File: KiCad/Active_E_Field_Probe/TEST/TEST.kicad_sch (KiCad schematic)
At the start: 91 parts

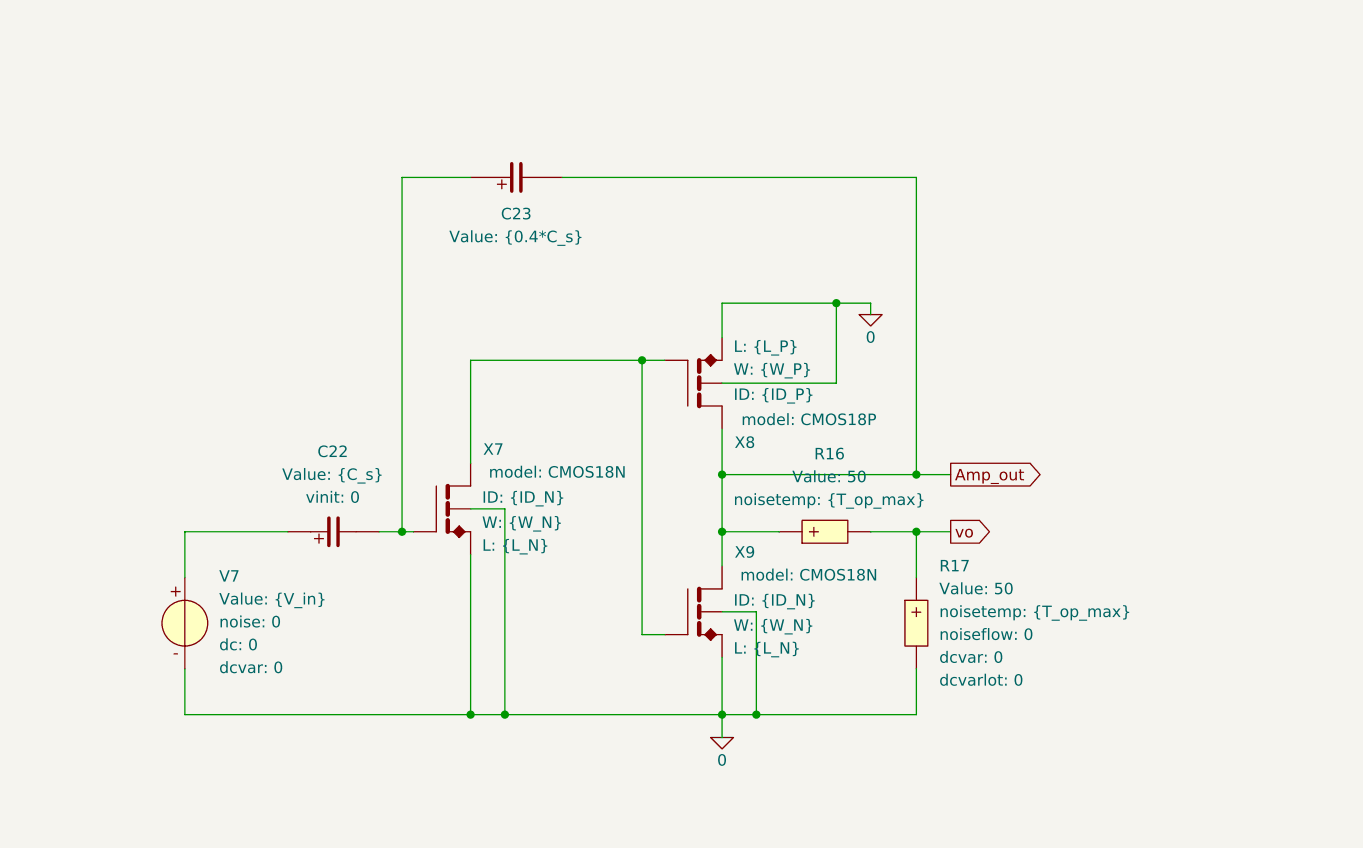
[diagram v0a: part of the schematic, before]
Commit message: something
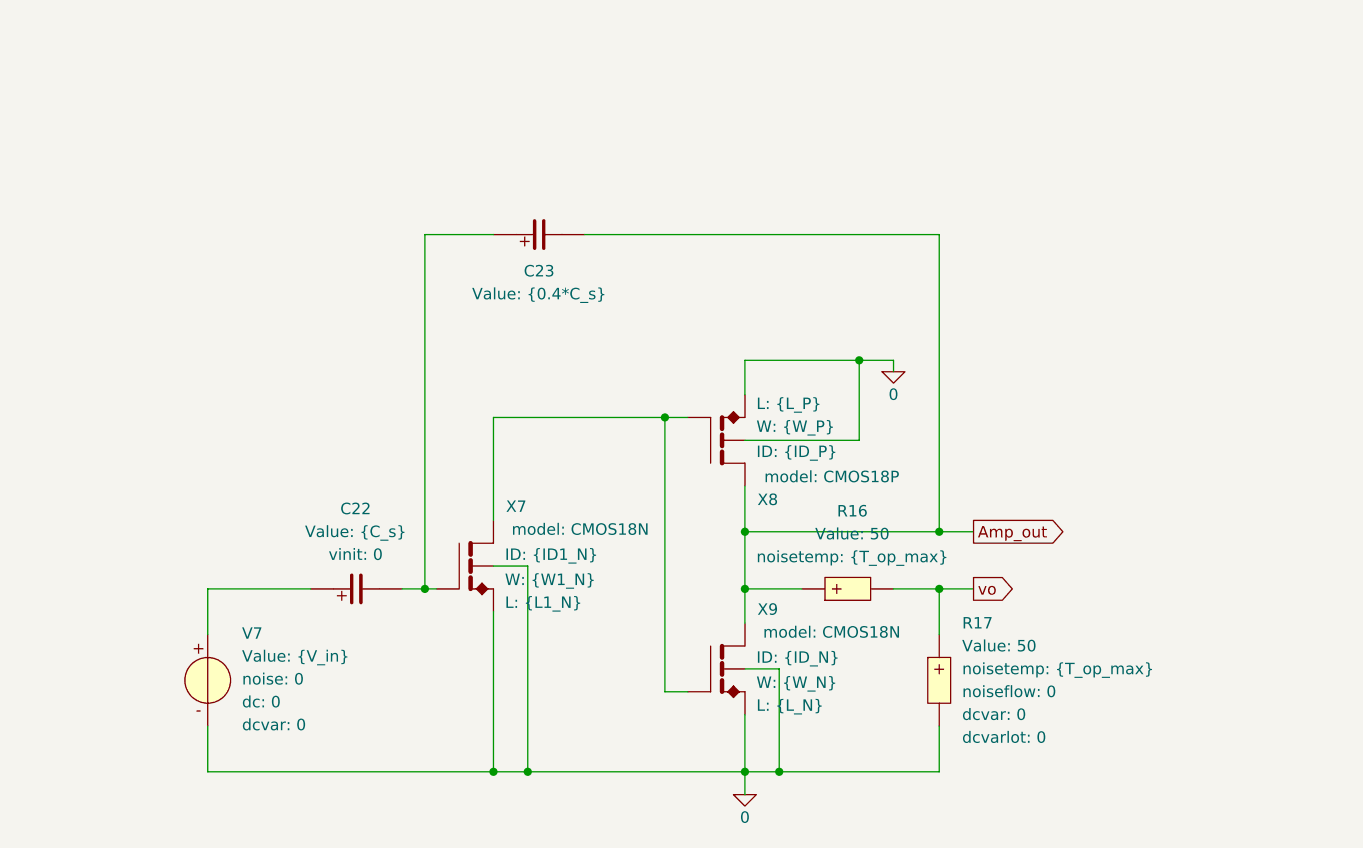
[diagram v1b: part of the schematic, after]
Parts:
- X7: ID {ID_N} -> {ID1_N}; L {L_N} -> {L1_N}; W {W_N} -> {W1_N}
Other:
- moved on the sheet: C22, C23, R16, R17

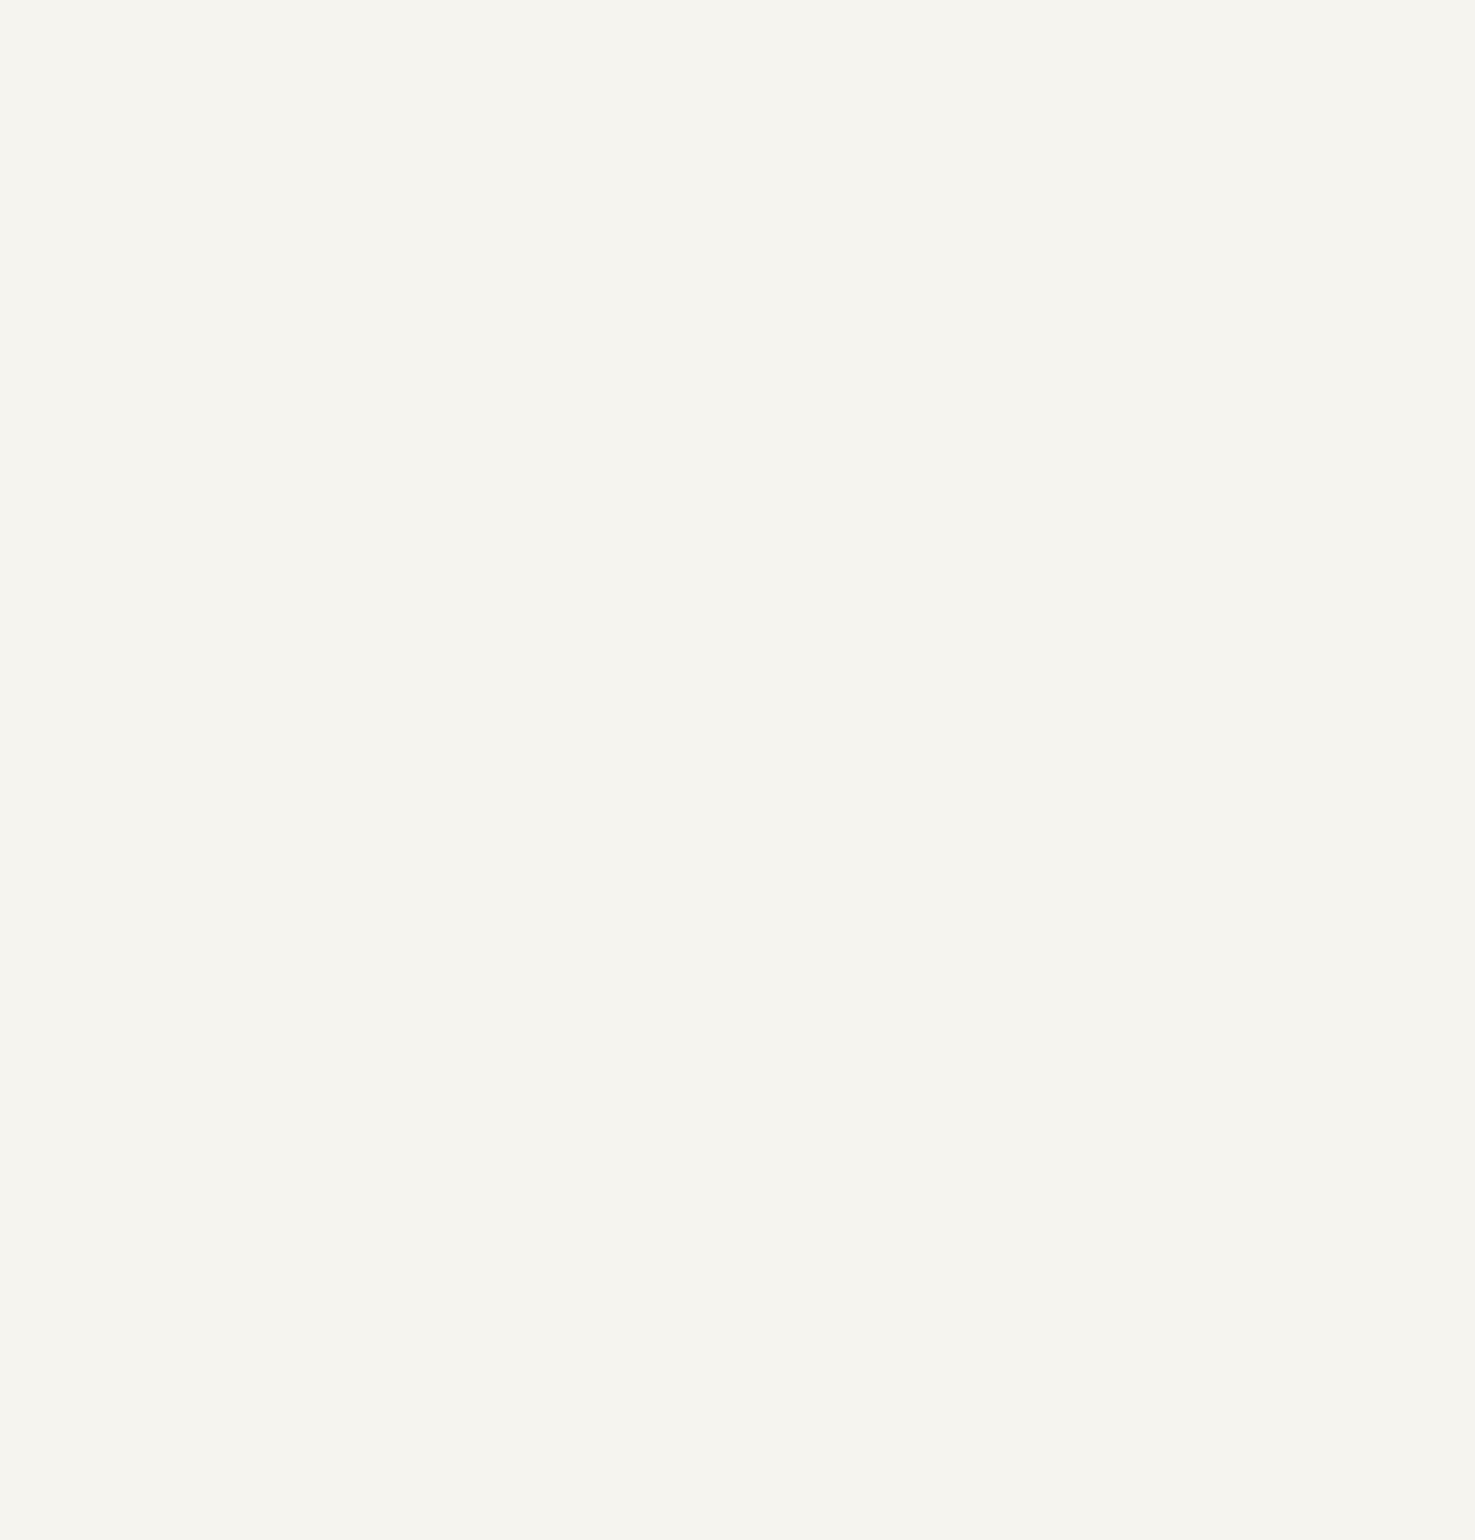
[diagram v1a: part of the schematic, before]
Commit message: Loopgain Fucked
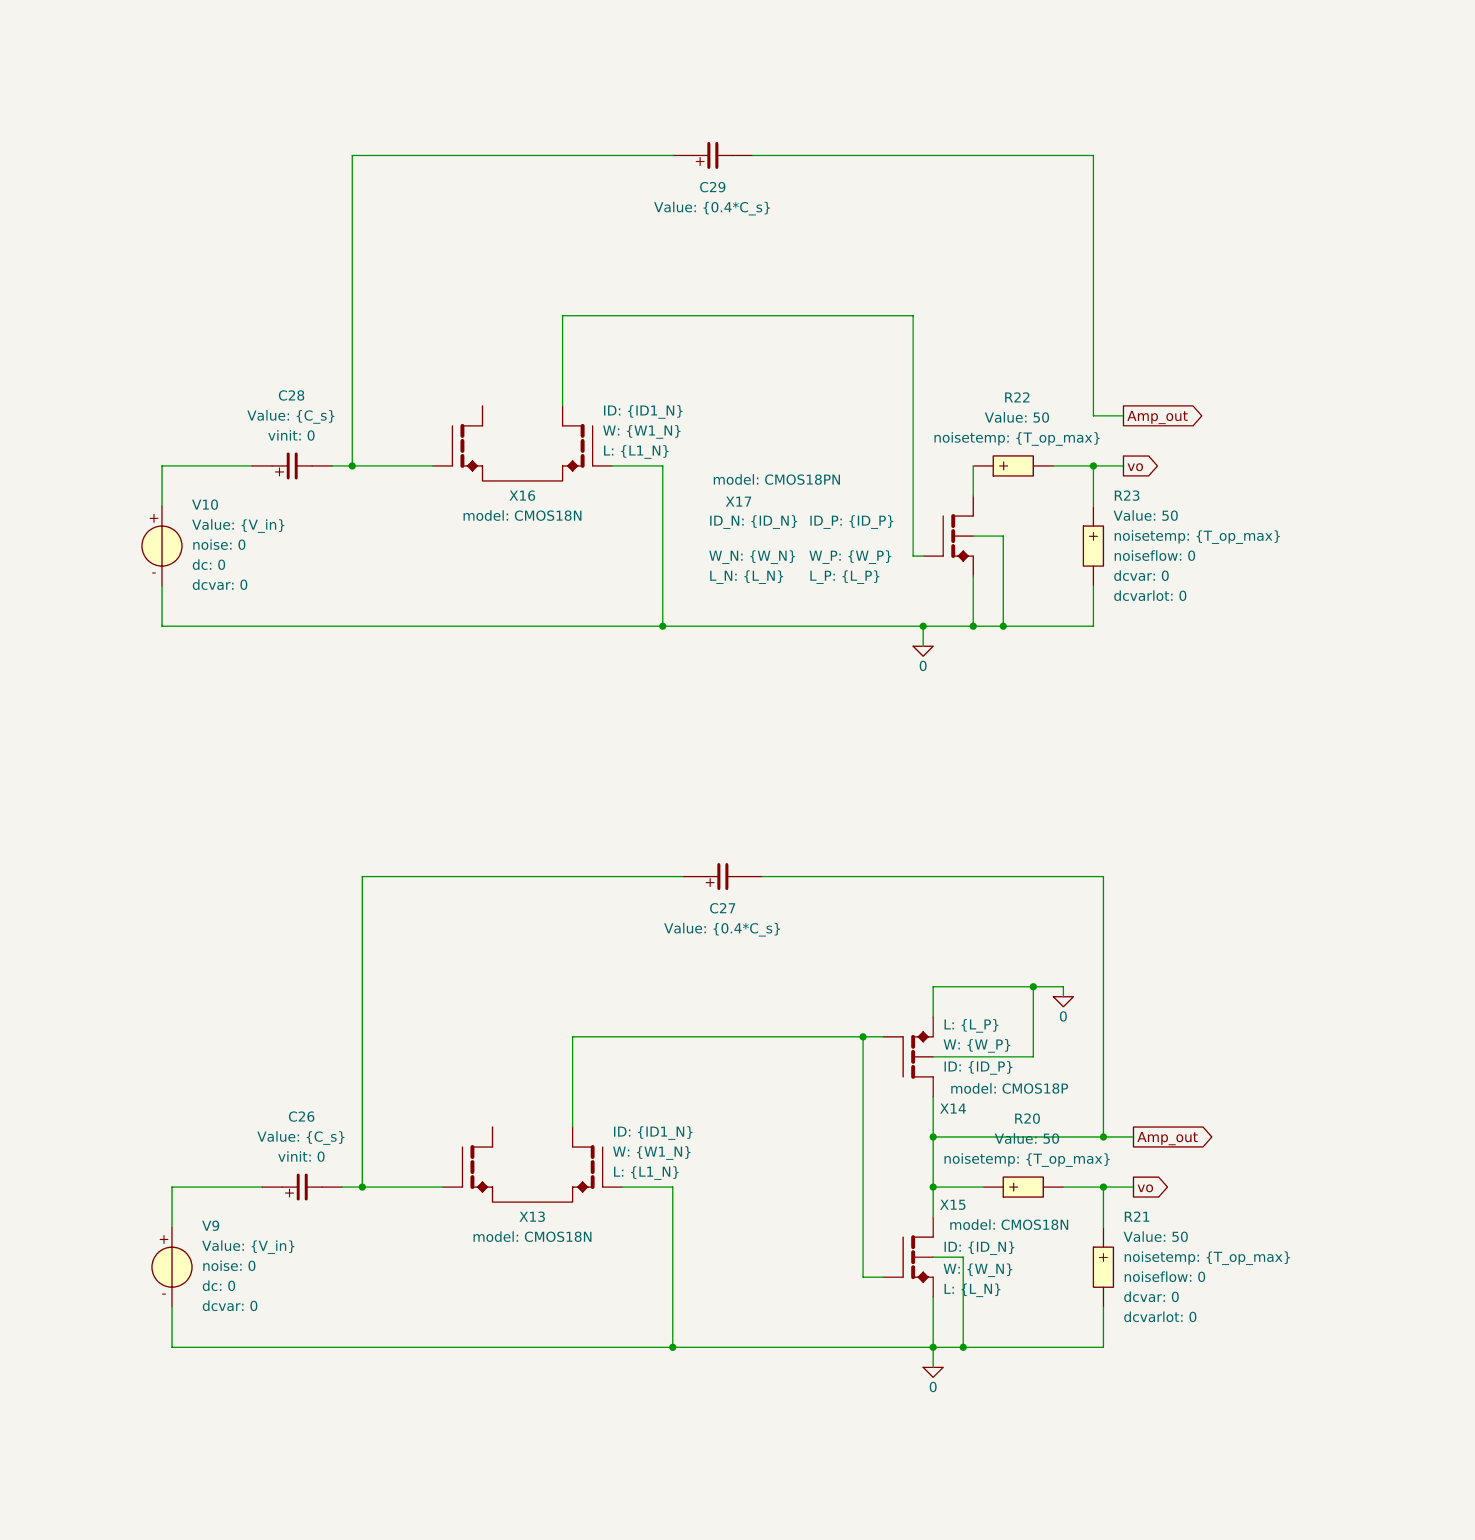
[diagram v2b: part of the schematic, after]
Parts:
- added C26, C28: {C_s}, symbol SLiCAP:C
- added C27, C29: {0.4*C_s}, symbol SLiCAP:C
- added R20, R21, R22, R23: 50, symbol SLiCAP:R
- added V10, V9: {V_in}, symbol SLiCAP:V
- added X13, X16: ~, symbol SLiCAP:XMD
- added X14, X15: ~, symbol SLiCAP:XM
- added X17: ~, symbol SLiCAP:XMPN
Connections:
- net 0: now also R21.2, R23.2, V10.2 (n), V9.2 (n), X13.4 (G2), X14.3 (S), X14.4 (B), X15.3 (S), X15.4 (B), X16.4 (G2), X17.3 (S), X17.4 (B)
- net Amp_out: now also C27.2, C29.2, R20.1, X14.1 (D), X15.1 (D)
- net vo: now also R20.2, R21.1, R22.2, R23.1
- new net: C28.2, C29.1, X16.3 (G1)
- new net: C28.1, V10.1 (p)
- new net: R22.1, X17.1 (D)
- new net: X16.2 (D2), X17.2 (G)
- new net: C26.1, V9.1 (p)
- new net: C26.2, C27.1, X13.3 (G1)
- new net: X13.2 (D2), X14.2 (G), X15.2 (G)
